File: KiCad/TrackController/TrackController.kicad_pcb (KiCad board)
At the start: 2 copper layers, 160 x 100 mm, 11 parts, among them J1 DE9_Plug_MountingHoles, SW1 SW_Push, SW2 SW_Push, U1 mini_esp32, U2 TXS0108EPW

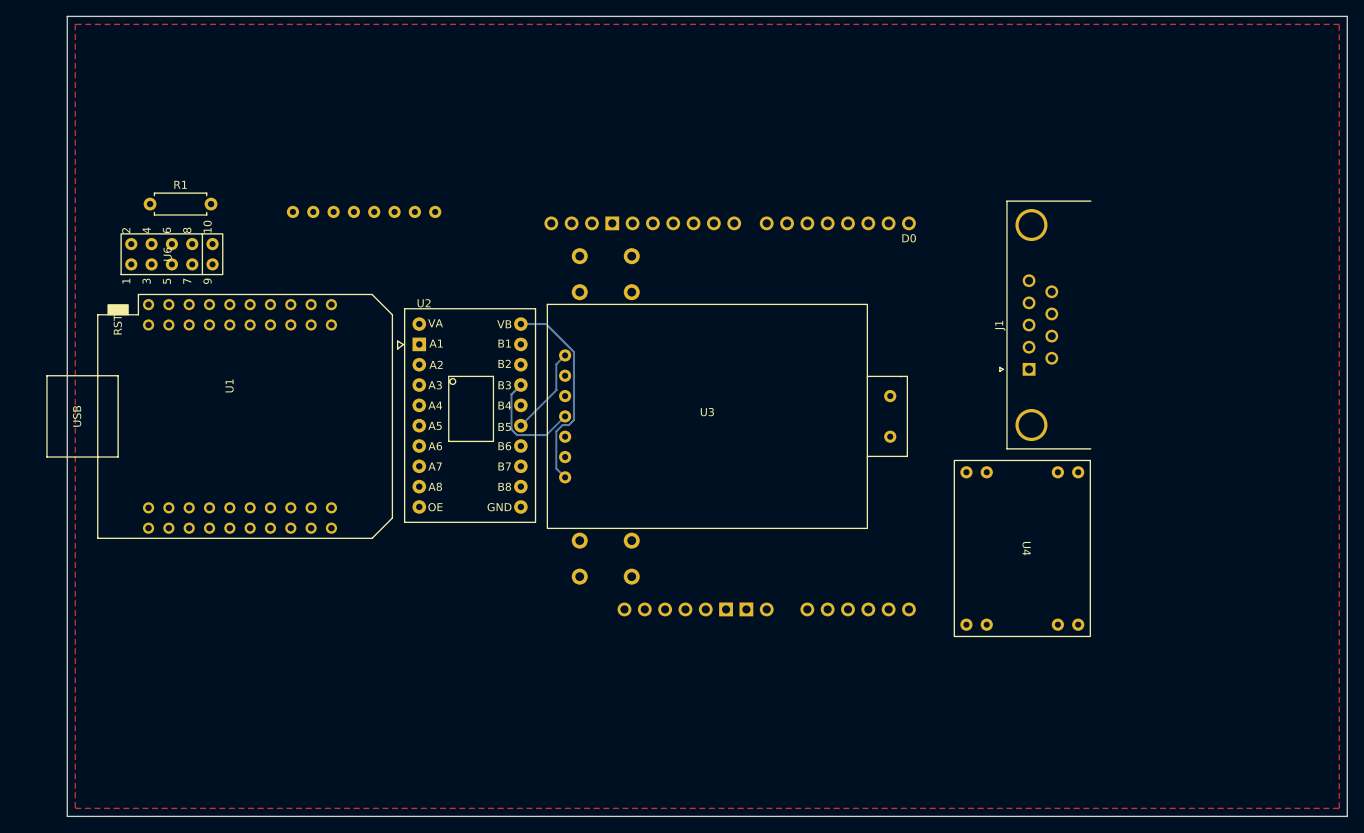
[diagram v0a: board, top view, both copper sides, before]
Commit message: 20240423
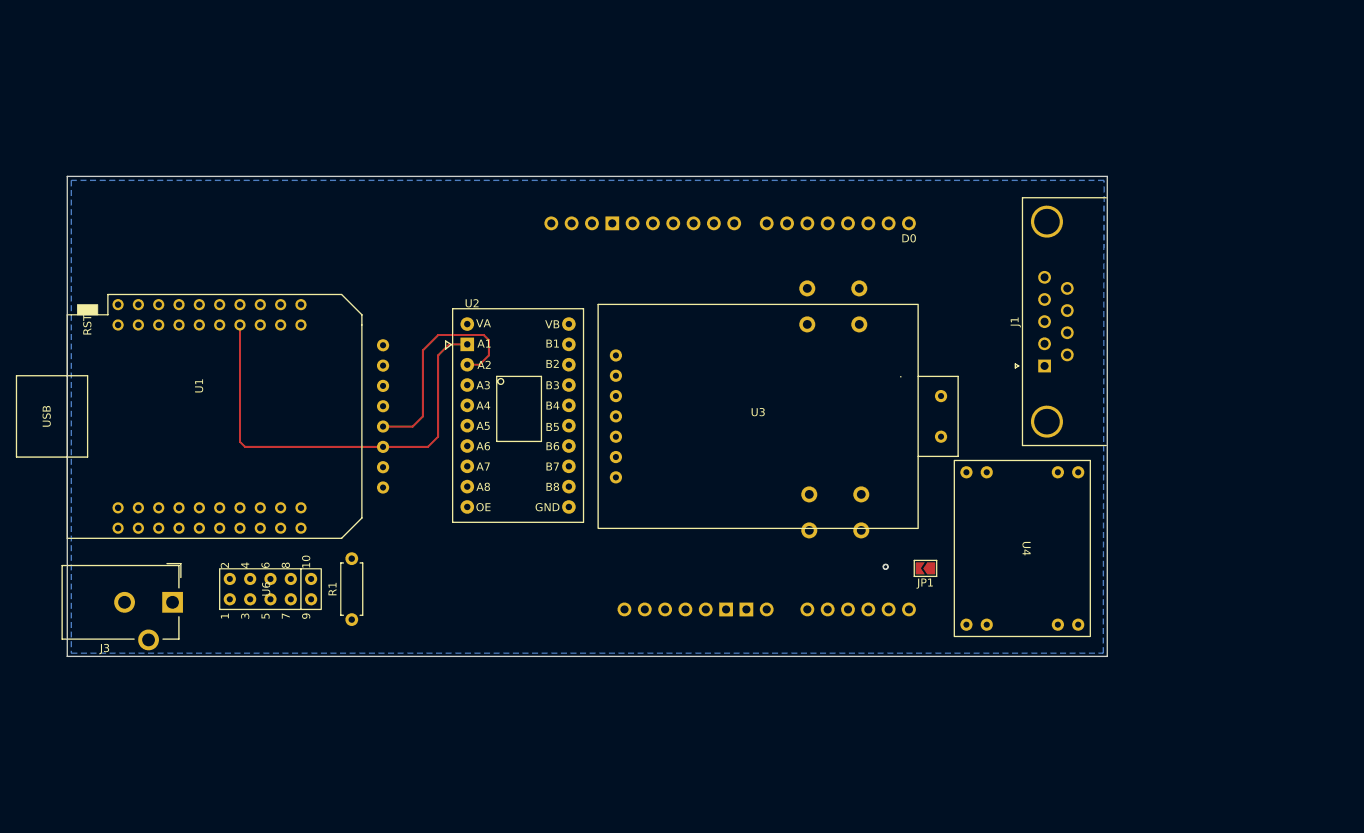
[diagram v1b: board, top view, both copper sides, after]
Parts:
- added J3: Barrel_Jack_Switch, Connector_BarrelJack:BarrelJack_CUI_PJ-102AH_Horizontal, F.Cu at (53.2, 123.2)
- added JP1: Jumper_2_Open, Jumper:SolderJumper-2_P1.3mm_Open_TrianglePad1.0x1.5mm, F.Cu at (147.3, 119.0)
- moved R1 57.7 mm to (75.6, 125.4), turned to 90 degrees
- moved U6 43.6 mm to (65.4, 121.6)
- moved SW1 29.3 mm to (132.8, 114.2)
- moved SW2 28.7 mm to (139.0, 84.0)
- moved LCD1 28.5 mm to (105.0, 100.0), turned to 0 degrees
- moved U3 6.35 mm to (126.4, 100.0)
- moved U2 6.00 mm to (90.0, 91.0)
- moved U1 3.81 mm to (57.8, 100.0)
- moved J1 1.98 mm to (162.2, 93.7)
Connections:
- SW2 pad 2: unconnected-(SW2-Pad2) -> /SPARE-SWITCH
- U1 pad 6: unconnected-(U1-IO_26/D0-Pad6) -> /SPARE-SWITCH
- U2 pad 10: unconnected-(U2-OE-Pad10) -> /3V3
- U2 pad 12: unconnected-(U2-B8-Pad12) -> /TRACK-PULSE-H-PROG-TTL
- U2 pad 13: unconnected-(U2-B7-Pad13) -> /TRACK-PULSE-H-TTL
- U2 pad 14: unconnected-(U2-B6-Pad14) -> /TRACK-ENABLE-TTL
- U2 pad 7: unconnected-(U2-A6-Pad7) -> /TRACK-POWER-ENABLE
- U2 pad 8: unconnected-(U2-A7-Pad8) -> /TRACK-PULSE-H
- U2 pad 9: unconnected-(U2-A8-Pad9) -> /TRACK-PULSE-H-PROG
- U5 pad J1-3: GND -> unconnected-(U5-AREF-PadJ1-3)
- U5 pad J1-4: (no net) -> GND
- U5 pad J1-5: unconnected-(U5-DIR-B-PadJ1-5) -> /TRACK-PULSE-H-PROG-TTL
- U5 pad J1-6: unconnected-(U5-DIR-A-PadJ1-6) -> /TRACK-PULSE-H-PROG
- U5 pad J1-7: unconnected-(U5-PWM-B-PadJ1-7) -> /TRACK-ENABLE-TTL
- U5 pad J1-9: (no net) -> unconnected-(U5-BREAK-A-PadJ1-9)
- U5 pad J2-5: unconnected-(U5-PWM-A-PadJ2-5) -> /TRACK-ENABLE-TTL
- U5 pad J4-1: unconnected-(U5-SENSE-A-PadJ4-1) -> /IS
- U6 pad 5: /iS -> /IS
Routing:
- net /SCK: track 0.00 -> 54.5 mm
- net /MOSI: track 0.00 -> 28.2 mm
- net /VCC: track 25.5 -> 0.00 mm, vias 0 -> 1
- net /SO-TTL: track 14.0 -> 0.00 mm
- net /CAN-INT-TTL*: track 11.1 -> 0.00 mm
- added copper zone on B.Cu, net GND
- removed copper zone on F.Cu, net GND
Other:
- board size 160 x 100 mm -> 130 x 60 mm
